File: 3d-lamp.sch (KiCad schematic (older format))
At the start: 22 parts, among them J1 USB, Q1 Q_NMOS_GDS, U1 ATTINY85-10SU

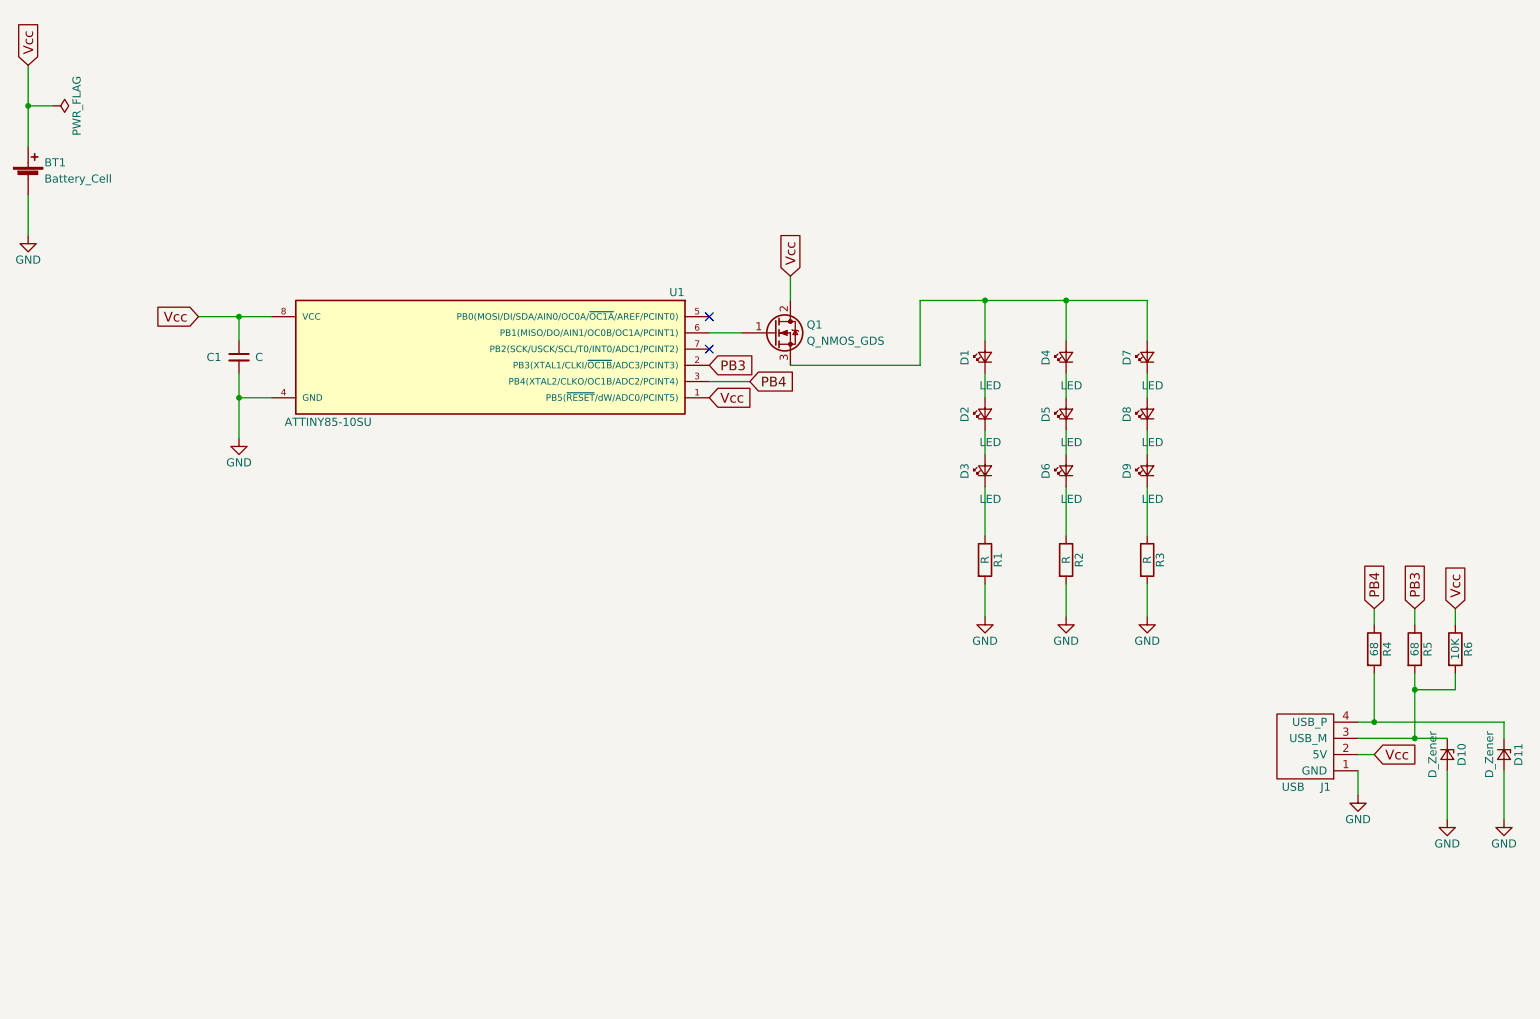
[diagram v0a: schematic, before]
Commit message: Schema fertiggestellt
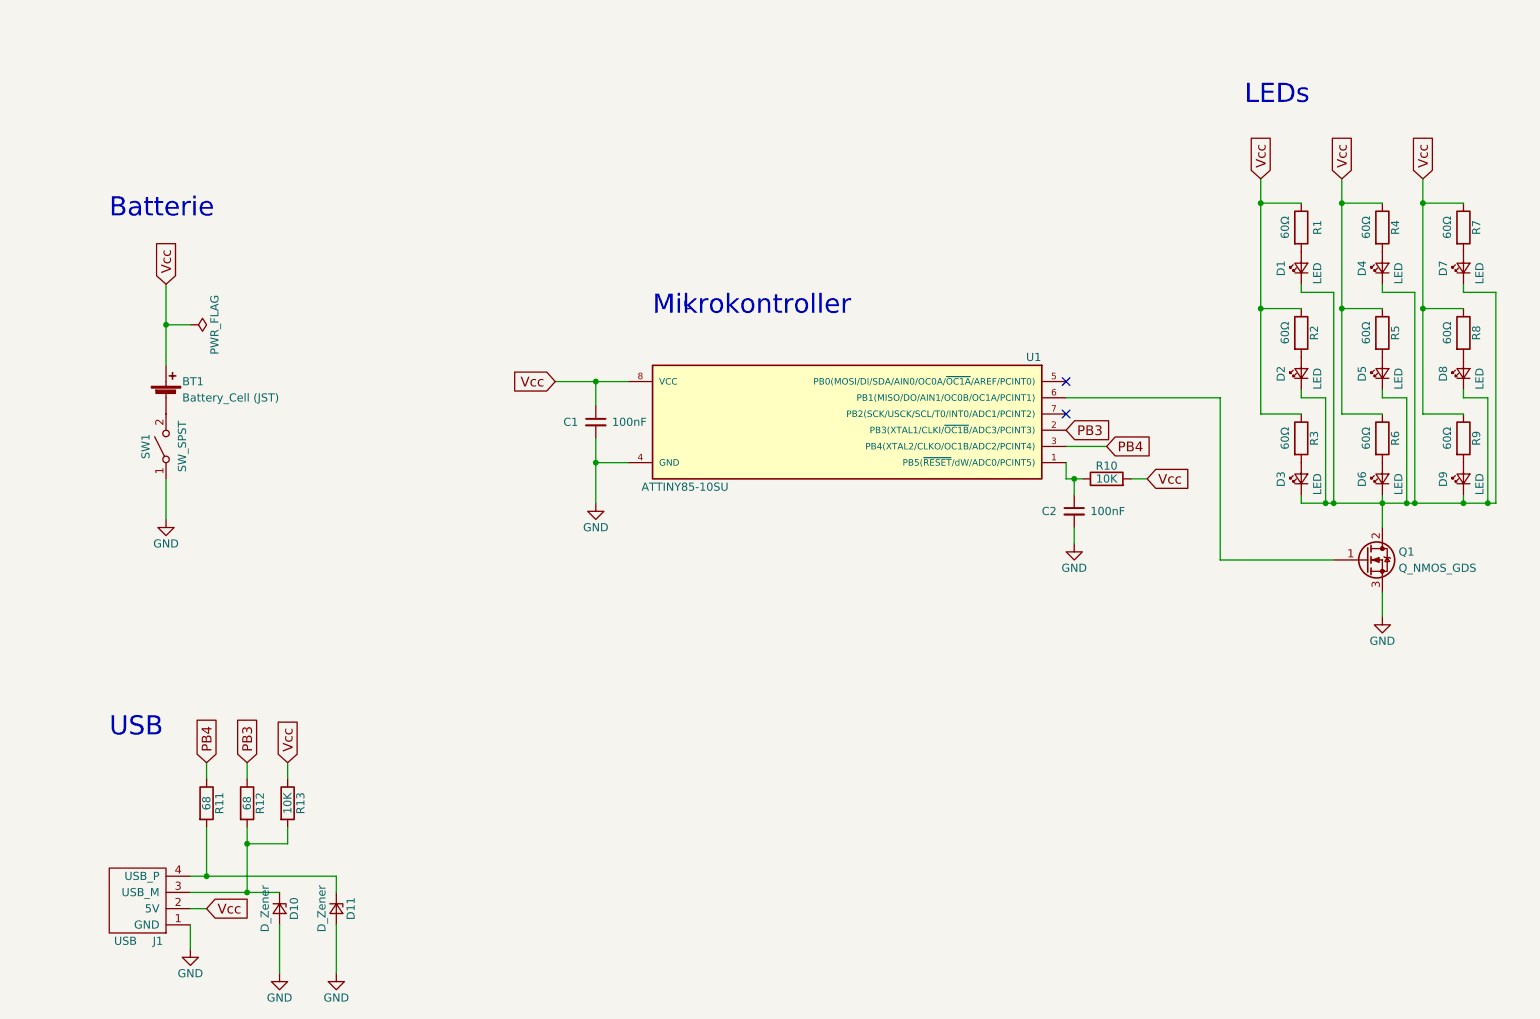
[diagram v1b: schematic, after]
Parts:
- removed R3: R, symbol R
- added C2: 100nF, symbol C_Small
- added R1, R4, R5, R6, R7, R8, R9: 60Ω, symbol R
- added R10: 10K, symbol R
- added SW1: SW_SPST, symbol SW_SPST
- BT1: value Battery_Cell -> Battery_Cell (JST)
- C1: value C -> 100nF
- R2: value R -> 60Ω
- R3: renamed from R1; value R -> 60Ω
- U1: Digikey (none) -> ATTINY85V-10SURCT-ND
- renumbered R4 to R11, R5 to R12, R6 to R13
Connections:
- net GND: now also Q1.3 (S), C2.2, SW1.1 (A); no longer BT1.2 (-), R2.2, R3.2
- net Vcc: now also R2.1, R3.1, R1.1, R10.2, R4.1, R5.1, R6.1, R7.1, R8.1, R9.1; no longer Q1.2 (D), U1.1 (PB5(~RESET~/dW/ADC0/PCINT5))
- net at D1.1 (K): now also D2.1 (K), D3.1 (K), D4.1 (K), D5.1 (K), D6.1 (K), D7.1 (K), D8.1 (K), D9.1 (K), Q1.2 (D); no longer D2.2 (A)
- net at D3.2 (A): now also R3.2; no longer D2.1 (K)
- net at D5.2 (A): now also R5.2; no longer D4.1 (K)
- net at D6.2 (A): now also R6.2; no longer D5.1 (K)
- net at D8.2 (A): now also R8.2; no longer D7.1 (K)
- net at D9.2 (A): now also R9.2; no longer D8.1 (K)
- new net: D1.2 (A), R1.2
- new net: D2.2 (A), R2.2
- new net: D4.2 (A), R4.2
- new net: D7.2 (A), R7.2
- new net: BT1.2 (-), SW1.2 (B)
- new net: C2.1, R10.1, U1.1 (PB5(~RESET~/dW/ADC0/PCINT5))
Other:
- note added: "Batterie"
- note added: "LEDs"
- note added: "Mikrokontroller"
- note added: "USB"
- moved on the sheet: BT1, C1, D1, D10, D11, D2, D3, D4, D5, D6, D7, D8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
